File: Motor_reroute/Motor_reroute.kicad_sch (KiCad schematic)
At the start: 36 parts, among them J11 Conn_01x03, J14 RJCSE538001, J17 874380843, J18 874380843, J2 RJCSE538001, J3 Conn_01x03, J7 Conn_01x05, J8 Conn_01x05

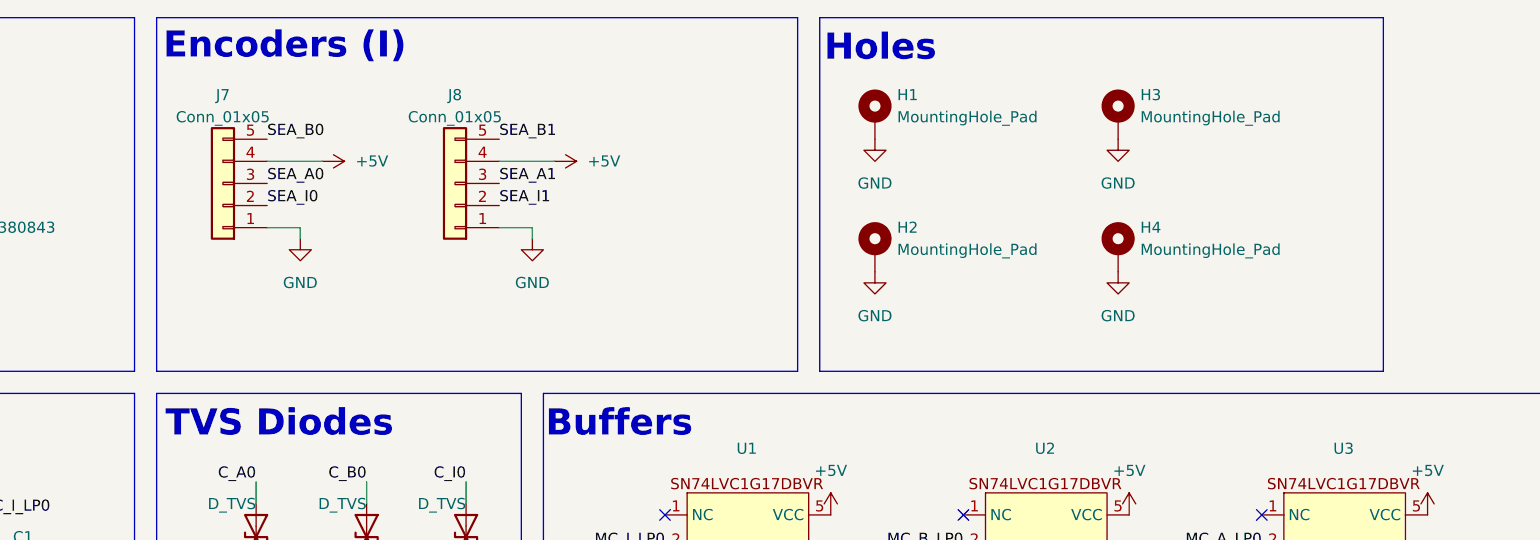
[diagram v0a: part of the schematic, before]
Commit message: added pcb updates
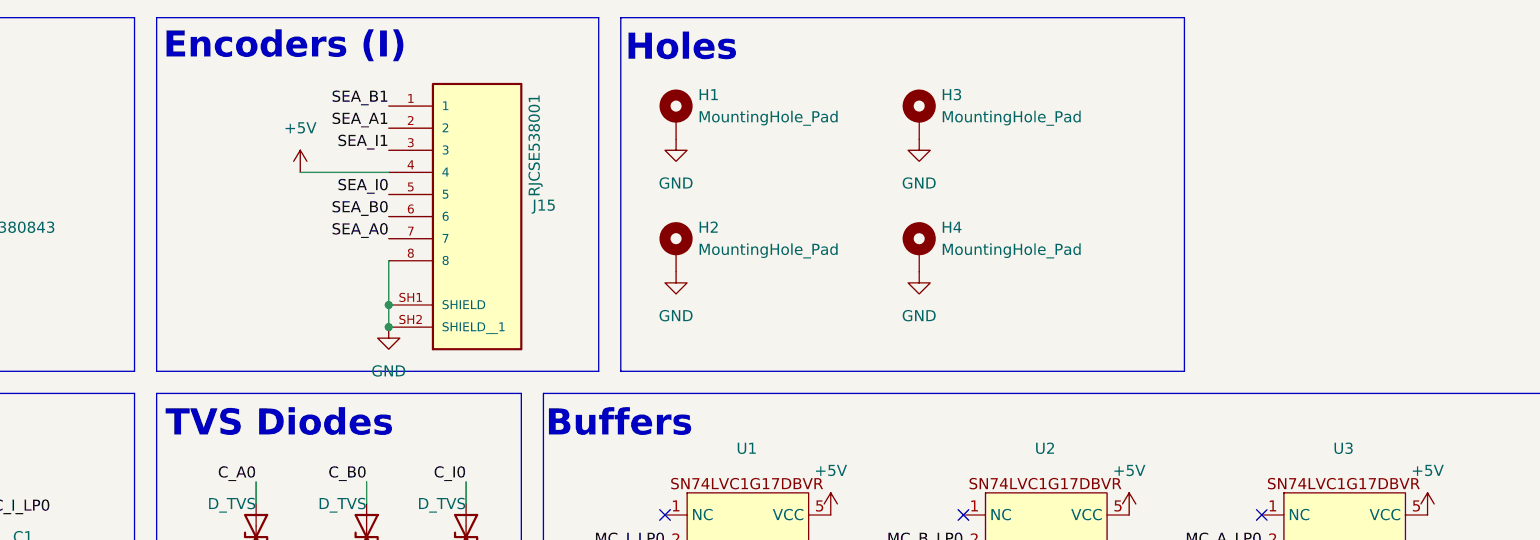
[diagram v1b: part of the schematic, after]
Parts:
- removed J7, J8: Conn_01x05, Connector_JST:JST_EH_B5B-EH-A_1x05_P2.50mm_Vertical, symbol Connector_Generic:Conn_01x05
- added J15: RJCSE538001, RJCSE538001:AMPHENOL_RJCSE538001, symbol RJCSE538001:RJCSE538001
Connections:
- net +5V: now also J15.4
- net GND: now also J15.8, J15.SH1 (SHIELD), J15.SH2 (SHIELD__1)
- net SEA_A0: now also J15.7
- net SEA_A1: now also J15.2
- net SEA_B0: now also J15.6
- net SEA_B1: now also J15.1
- net SEA_I0: now also J15.5
- net SEA_I1: now also J15.3
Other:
- moved on the sheet: H1, H2, H3, H4
